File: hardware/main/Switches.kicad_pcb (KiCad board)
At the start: 4 copper layers, 120 x 75 mm, 108 parts, among them J101 BusBar, J102 BusBar, J103 BusBar, J104 BusBar, J105 Conn_02x03_Odd_Even, Q101 IPT015N10N5, Q102 IPT015N10N5, Q103 IPT015N10N5, Q104 IPT015N10N5, Q105 IPT015N10N5, Q106 IPT015N10N5, Q107 IPT015N10N5, Q108 IPT015N10N5, Q109 IPT015N10N5, Q110 IPT015N10N5, Q111 IPT015N10N5, Q112 IPT015N10N5, U101 UCC27211DDAR, U102 UCC27211DDAR

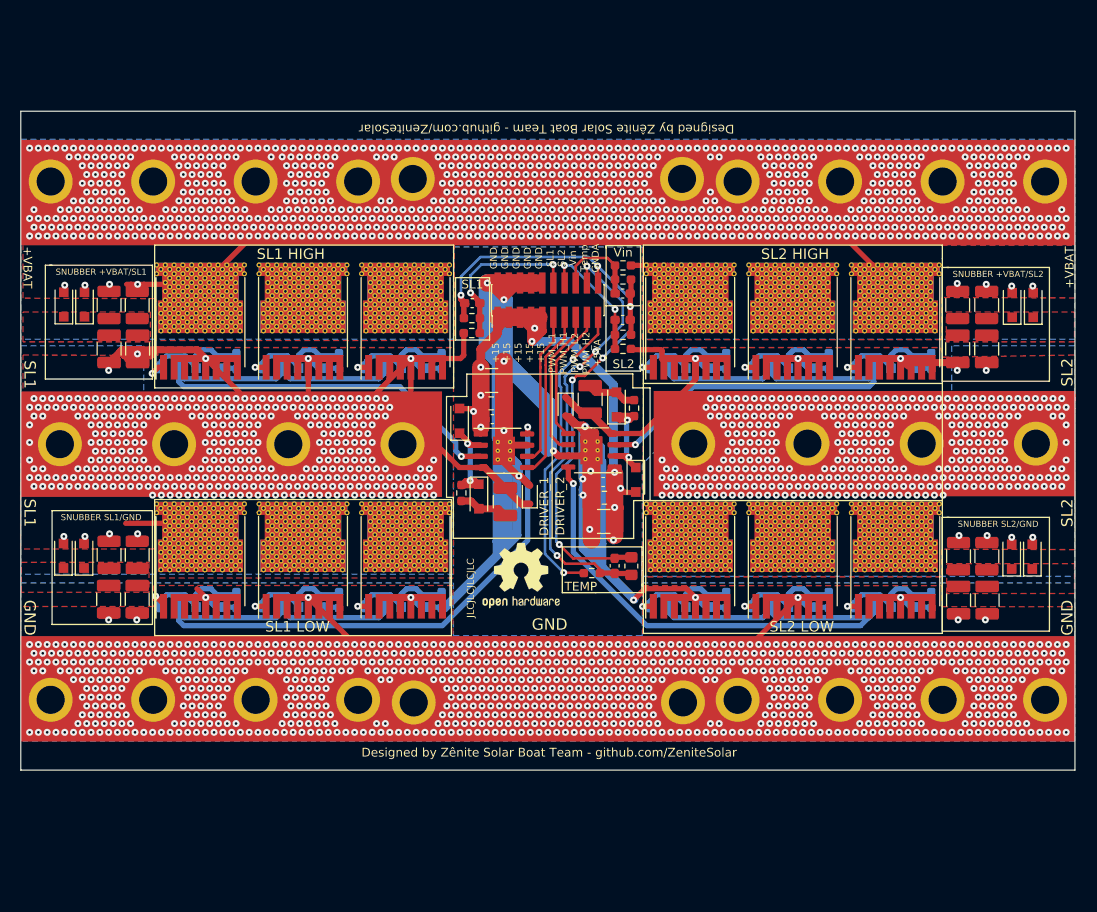
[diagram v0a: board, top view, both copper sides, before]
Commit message: board finalized
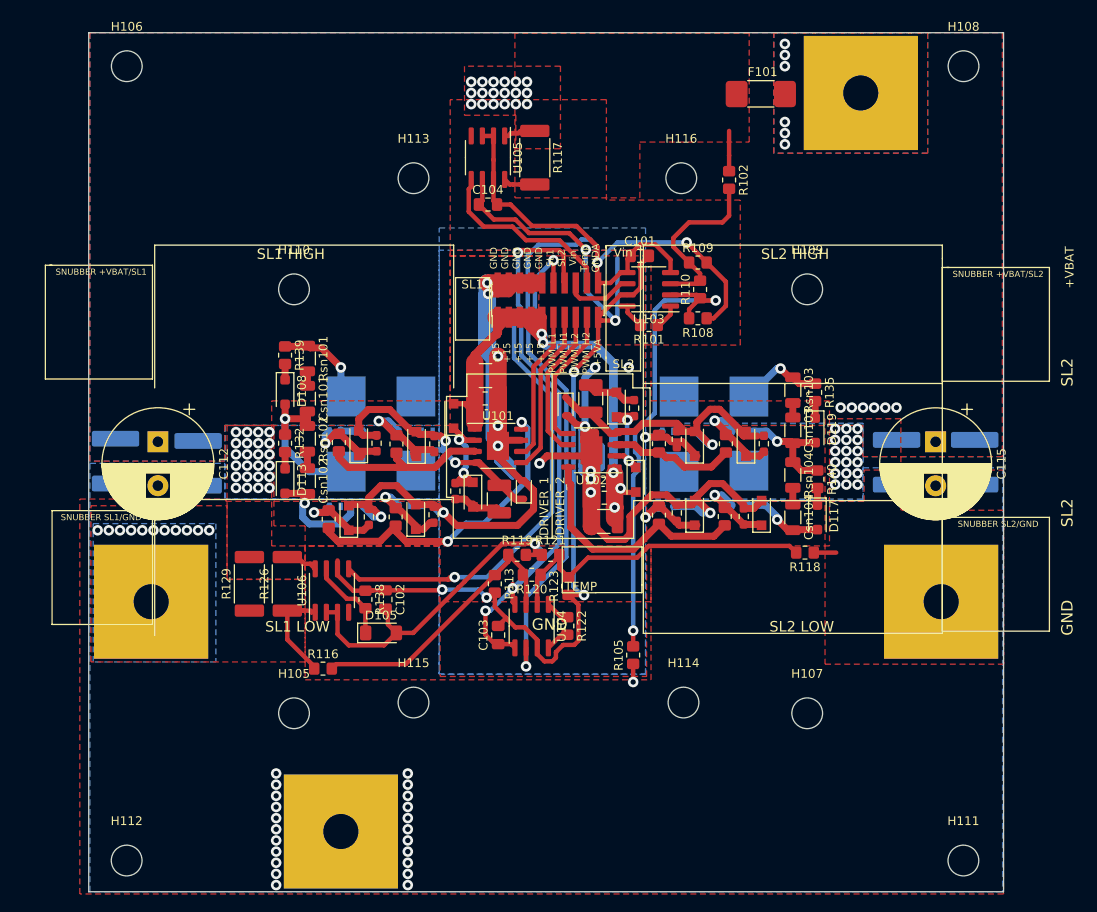
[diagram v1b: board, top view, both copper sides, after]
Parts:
- removed C131, C132, C133: 1n, Capacitor_SMD:C_0603_1608Metric_Pad1.08x0.95mm_HandSolder
- removed C134: 100n, Capacitor_SMD:C_0603_1608Metric_Pad1.08x0.95mm_HandSolder
- removed Csn105, Csn107: 100n, Capacitor_SMD:C_1210_3225Metric_Pad1.33x2.70mm_HandSolder
- removed Csn106, Csn108: NC, Capacitor_SMD:C_1210_3225Metric_Pad1.33x2.70mm_HandSolder
- removed Dsn101, Dsn103, Dsn105, Dsn107: MBR2H100SFT3G, Diode_SMD:D_SOD-123F
- removed Dsn102, Dsn104, Dsn106, Dsn108: NC, Diode_SMD:D_SOD-123F
- removed J101, J102: BusBar, Switches:BusBar1
- removed J103, J104: BusBar, Switches:BusBar2
- removed Q103, Q106, Q109, Q112: IPT015N10N5, Switches:Infineon_PG-HSOF-8-1_ThermalVias3
- removed REF**: OSHW-Logo2_9.8x8mm_SilkScreen, Symbol:OSHW-Logo2_9.8x8mm_SilkScreen
- removed Rsn105, Rsn107: 10, Resistor_SMD:R_1210_3225Metric_Pad1.30x2.65mm_HandSolder
- removed Rsn106, Rsn108: NC, Resistor_SMD:R_1210_3225Metric_Pad1.30x2.65mm_HandSolder
- removed TH101: SDNT2012X103F3950FTF, Resistor_SMD:R_0805_2012Metric_Pad1.20x1.40mm_HandSolder
- added C101: 100n, Capacitor_SMD:C_0805_2012Metric_Pad1.18x1.45mm_HandSolder, F.Cu at (172.7, 80.0)
- added C102: 100n, Capacitor_SMD:C_0805_2012Metric_Pad1.18x1.45mm_HandSolder, F.Cu at (143.8, 119.1)
- added C103: 100n, Capacitor_SMD:C_0805_2012Metric_Pad1.18x1.45mm_HandSolder, F.Cu at (156.6, 123.2)
- added C104: 100n, Capacitor_SMD:C_0805_2012Metric_Pad1.18x1.45mm_HandSolder, F.Cu at (155.4, 74.2)
- added C112: 80V 4700uF, Capacitor_THT:CP_Radial_D12.5mm_P5.00mm, F.Cu at (117.9, 101.2)
- added C115: 80V 4700uF, Capacitor_THT:CP_Radial_D12.5mm_P5.00mm, F.Cu at (206.4, 101.2)
- added Cc101: 250V 1uF X7R ±10% 20mR 2220, Capacitor_SMD:C_2220_5650Metric, B.Cu at (201.9, 103.5)
- added Cc102: 250V 1uF X7R ±10% 20mR 2220, Capacitor_SMD:C_2220_5650Metric, B.Cu at (210.8, 103.5)
- added Cc103: 250V 1uF X7R ±10% 20mR 2220, Capacitor_SMD:C_2220_5650Metric, B.Cu at (122.4, 103.6)
- added Cc104: 250V 1uF X7R ±10% 20mR 2220, Capacitor_SMD:C_2220_5650Metric, B.Cu at (113.0, 103.4)
- added D119: SMF100A, Diode_SMD:D_SOD-123F, F.Cu at (192.7, 99.9)
- added F101: 65V 20A 3mOhms Fuse, Zenite:S6125-F, F.Cu at (186.7, 61.5)
- added H101: Vin+, Zenite:MountingHole_13mmx13mm_Rectangular, F.Cu at (197.9, 61.5)
- added H102: Vin-, Zenite:MountingHole_13mmx13mm_Rectangular, F.Cu at (138.7, 145.5)
- added H103: Vout-, Zenite:MountingHole_13mmx13mm_Rectangular, F.Cu at (207.0, 119.4)
- added H104: Vout+, Zenite:MountingHole_13mmx13mm_Rectangular, F.Cu at (117.1, 119.4)
- added H105: MountingHole, MountingHole:MountingHole_3.5mm, F.Cu at (133.3, 132.1)
- added H106: MountingHole, MountingHole:MountingHole_3.5mm, F.Cu at (114.3, 58.4)
- added H107: MountingHole, MountingHole:MountingHole_3.5mm, F.Cu at (191.8, 132.1)
- added H108: MountingHole, MountingHole:MountingHole_3.5mm, F.Cu at (209.6, 58.4)
- added H109: MountingHole, MountingHole:MountingHole_3.5mm, F.Cu at (191.8, 83.8)
- added H110: MountingHole, MountingHole:MountingHole_3.5mm, F.Cu at (133.3, 83.8)
- added H111: MountingHole, MountingHole:MountingHole_3.5mm, F.Cu at (209.6, 148.8)
- added H112: MountingHole, MountingHole:MountingHole_3.5mm, F.Cu at (114.3, 148.8)
- added H113: MountingHole, MountingHole:MountingHole_3.5mm, F.Cu at (147.0, 71.2)
- added H114: MountingHole, MountingHole:MountingHole_3.5mm, F.Cu at (177.7, 130.9)
- added H115: MountingHole, MountingHole:MountingHole_3.5mm, F.Cu at (147.0, 130.9)
- added H116: MountingHole, MountingHole:MountingHole_3.5mm, F.Cu at (177.4, 71.2)
- added R101: ?, Resistor_SMD:R_0805_2012Metric_Pad1.20x1.40mm_HandSolder, F.Cu at (173.8, 87.9)
- added R102: ?, Resistor_SMD:R_0805_2012Metric_Pad1.20x1.40mm_HandSolder, F.Cu at (182.9, 71.4)
- added R109: ?, Resistor_SMD:R_0805_2012Metric_Pad1.20x1.40mm_HandSolder, F.Cu at (179.3, 80.8)
- added R110: ?, Resistor_SMD:R_0805_2012Metric_Pad1.20x1.40mm_HandSolder, F.Cu at (179.6, 83.8)
- added R138: 1k, Resistor_SMD:R_0805_2012Metric_Pad1.20x1.40mm_HandSolder, F.Cu at (141.5, 119.1)
- added R139: 0R, Resistor_SMD:R_0805_2012Metric_Pad1.20x1.40mm_HandSolder, F.Cu at (132.3, 91.3)
- added R140: 0R, Resistor_SMD:R_0805_2012Metric_Pad1.20x1.40mm_HandSolder, F.Cu at (192.9, 105.4)
- added U103: INA823, Package_SO:SOIC-8_3.9x4.9mm_P1.27mm, F.Cu at (173.7, 83.8)
- added U104: INA823, Package_SO:SOIC-8_3.9x4.9mm_P1.27mm, F.Cu at (160.4, 122.2)
- added U105: INA283, Package_SO:SOIC-8_3.9x4.9mm_P1.27mm, F.Cu at (155.4, 68.8)
- added U106: INA283, Package_SO:SOIC-8_3.9x4.9mm_P1.27mm, F.Cu at (137.7, 118.1)
- Csn101, Csn103: footprint Capacitor_SMD:C_1210_3225Metric_Pad1.33x2.70mm_HandSolder -> Resistor_SMD:R_1206_3216Metric
- Csn102, Csn104: value NC -> 100n; footprint Capacitor_SMD:C_1210_3225Metric_Pad1.33x2.70mm_HandSolder -> Resistor_SMD:R_1206_3216Metric
- D101, D104, D106, D107, D109, D112, D115, D116, R103, R104, R106, R107, R111, R112, R114, R115, R124, R125, R127, R128, R130, R131, R133, R134: moved to F.Cu
- D105: value B0530W -> 3v6; footprint Diode_SMD:D_SOD-123F -> Diode_SMD:D_MiniMELF; moved to F.Cu
- D108, D113, D117: value B0530W -> SMF100A; moved to F.Cu
- Q101, Q102, Q104, Q105, Q107, Q108, Q110, Q111: value IPT015N10N5 -> BSC093N15NS5; footprint Switches:Infineon_PG-HSOF-8-1_ThermalVias3 -> Zenite:TDSON-8-3; moved to B.Cu
- R105, R108, R113, R116: value 4R7 -> ?; moved to F.Cu
- R117: value 5k6 -> 1.0mR 1% 5W 50ppm; footprint Resistor_SMD:R_0603_1608Metric_Pad0.98x0.95mm_HandSolder -> Resistor_SMD:R_2512_6332Metric_Pad1.40x3.35mm_HandSolder
- R118, R119, R120: value 10k -> ?; footprint Resistor_SMD:R_0603_1608Metric_Pad0.98x0.95mm_HandSolder -> Resistor_SMD:R_0805_2012Metric_Pad1.20x1.40mm_HandSolder
- R121: value 330 -> ?; footprint Resistor_SMD:R_0603_1608Metric_Pad0.98x0.95mm_HandSolder -> Resistor_SMD:R_0805_2012Metric_Pad1.20x1.40mm_HandSolder
- R122, R123: value 3k3 -> ?; footprint Resistor_SMD:R_0603_1608Metric_Pad0.98x0.95mm_HandSolder -> Resistor_SMD:R_0805_2012Metric_Pad1.20x1.40mm_HandSolder
- R126, R129: value 10k -> 1.0mR 1% 5W 50ppm; footprint Resistor_SMD:R_0603_1608Metric_Pad0.98x0.95mm_HandSolder -> Resistor_SMD:R_2512_6332Metric_Pad1.40x3.35mm_HandSolder; moved to F.Cu
- R132, R135: value 10k -> 0R; footprint Resistor_SMD:R_0603_1608Metric_Pad0.98x0.95mm_HandSolder -> Resistor_SMD:R_0805_2012Metric_Pad1.20x1.40mm_HandSolder; moved to F.Cu
- Rsn101, Rsn103: footprint Resistor_SMD:R_1210_3225Metric_Pad1.30x2.65mm_HandSolder -> Resistor_SMD:R_1206_3216Metric
- Rsn102, Rsn104: value NC -> 10; footprint Resistor_SMD:R_1210_3225Metric_Pad1.30x2.65mm_HandSolder -> Resistor_SMD:R_1206_3216Metric
- U101, U102: footprint Switches:SOIC-8-1EP_3.9x4.9mm_P1.27mm_EP2.514x3.2mm_ThermalVias -> Package_SO:SOIC-8-1EP_3.9x4.9mm_P1.27mm_EP2.514x3.2mm
- moved R132 74.2 mm to (132.3, 101.3), turned to -90 degrees
- moved D113 71.5 mm to (132.3, 105.6), turned to -90 degrees
- moved R116 62.1 mm to (136.7, 127.0)
- moved R108 49.2 mm to (179.3, 87.1), turned to 180 degrees
- moved R113 48.8 mm to (156.2, 117.3), turned to -90 degrees
- moved R117 47.7 mm to (160.8, 68.8), turned to -90 degrees
- moved R118 45.4 mm to (191.5, 113.8), turned to 180 degrees
- moved R105 44.0 mm to (172.0, 125.5), turned to 90 degrees
- moved R120 36.7 mm to (160.4, 116.3)
- moved R123 35.4 mm to (164.6, 117.6), turned to 90 degrees
- moved R122 33.7 mm to (164.5, 122.1), turned to -90 degrees
- moved R126 30.8 mm to (132.6, 117.3)
- moved D105 30.4 mm to (143.3, 122.9)
- moved Rsn104 29.3 mm to (190.1, 105.0)
- moved Csn104 29.2 mm to (190.1, 109.8)
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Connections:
- Csn102 pad 1: Net-(Csn101-Pad1) -> Net-(Csn102-Pad1)
- Csn102 pad 2: /SL1 -> GND
- Csn104 pad 1: Net-(Csn103-Pad1) -> Net-(Csn104-Pad1)
- Csn104 pad 2: /SL2 -> GND
- D105 pad 1: /GH1_3 -> Net-(D105-K)
- D105 pad 2: /SL1 -> GNDA
- D108 pad 1: /GL1_3 -> Net-(D108-A1)
- D108 pad 2: GND -> /SL1
- D113 pad 1: /GH2_3 -> Net-(D113-A1)
- D113 pad 2: /SL2 -> GND
- D117 pad 1: /GL3_3 -> Net-(D117-A1)
- J105 pad 12: /SL1_sen -> /Vout_Sense
- J105 pad 14: /SL2_sen -> /Iout_Sense
- J105 pad 16: /Vin_sen -> /Vin_Sense
- J105 pad 18: /TEMP1 -> /Iin_Sense
- Q101 pad 2: /SL1 -> +BATT
- Q101 pad 3: +BATT -> /SL1
- Q102 pad 2: /SL1 -> +BATT
- Q102 pad 3: +BATT -> /SL1
- Q104 pad 2: /SL2 -> +BATT
- Q104 pad 3: +BATT -> /SL2
- Q105 pad 2: /SL2 -> +BATT
- Q105 pad 3: +BATT -> /SL2
- Q107 pad 2: GND -> /SL1
- Q107 pad 3: /SL1 -> GND
- Q108 pad 2: GND -> /SL1
- Q108 pad 3: /SL1 -> GND
- Q110 pad 2: GND -> /SL2
- Q110 pad 3: /SL2 -> GND
- Q111 pad 2: GND -> /SL2
- Q111 pad 3: /SL2 -> GND
- R103 pad 2: Net-(R103-Pad2) -> Net-(U101-HO)
- R104 pad 2: Net-(R103-Pad2) -> Net-(U101-HO)
- R105 pad 1: /GH1_3 -> GND
- R105 pad 2: Net-(R103-Pad2) -> Net-(U103--)
- R106 pad 2: Net-(R106-Pad2) -> Net-(U101-LO)
- R107 pad 2: Net-(R106-Pad2) -> Net-(U101-LO)
- R108 pad 1: /GL1_3 -> GNDA
- R108 pad 2: Net-(R106-Pad2) -> Net-(U103--)
- R111 pad 2: Net-(R111-Pad2) -> Net-(U102-HO)
- R112 pad 2: Net-(R111-Pad2) -> Net-(U102-HO)
- R113 pad 1: /GH2_3 -> Net-(U104-+)
- R113 pad 2: Net-(R111-Pad2) -> +5VA
- R114 pad 2: Net-(R114-Pad2) -> Net-(U102-LO)
- R115 pad 2: Net-(R114-Pad2) -> Net-(U102-LO)
- R116 pad 1: /GL3_3 -> /Vout+
- R116 pad 2: Net-(R114-Pad2) -> Net-(U104-+)
- R117 pad 1: +5VA -> +BATT
- R117 pad 2: /TEMP1 -> /Vbat+_Fus
- R118 pad 1: /SL1 -> /SL2
- R118 pad 2: /SL1_sen -> Net-(U104--)
- R119 pad 1: /SL2 -> Net-(U104-+)
- R119 pad 2: /SL2_sen -> GNDA
- R120 pad 1: +BATT -> Net-(U104--)
- R120 pad 2: /Vin_sen -> Net-(U104-+)
- R121 pad 1: /SL1_sen -> GNDA
- R121 pad 2: GNDA -> Net-(U104--)
- R122 pad 1: /SL2_sen -> Net-(R122-Pad1)
- R122 pad 2: GNDA -> Net-(R122-Pad2)
- R123 pad 1: /Vin_sen -> +5VA
- R123 pad 2: GNDA -> Net-(U104--)
- R126 pad 1: /SL1 -> /Vout+
- R126 pad 2: /GH1_3 -> /SL1
- R129 pad 1: GND -> /Vout+
- R129 pad 2: /GL1_3 -> /SL1
- R132 pad 1: /SL2 -> /SL1
- R132 pad 2: /GH2_3 -> Net-(D113-A1)
- R135 pad 1: GND -> +BATT
- R135 pad 2: /GL3_3 -> Net-(D119-A1)
- Rsn102 pad 1: +BATT -> /SL1
- Rsn102 pad 2: Net-(Csn101-Pad1) -> Net-(Csn102-Pad1)
- Rsn104 pad 1: +BATT -> /SL2
- Rsn104 pad 2: Net-(Csn103-Pad1) -> Net-(Csn104-Pad1)
- U101 pad 3: Net-(R103-Pad2) -> Net-(U101-HO)
- U101 pad 8: Net-(R106-Pad2) -> Net-(U101-LO)
- U102 pad 3: Net-(R111-Pad2) -> Net-(U102-HO)
- U102 pad 8: Net-(R114-Pad2) -> Net-(U102-LO)
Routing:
- net GND: track 392.4 -> 287.5 mm, vias 974 -> 40
- net GNDA: track 77.9 -> 176.5 mm, vias 6 -> 5
- net +5VA: track 34.9 -> 127.0 mm, vias 2 -> 6
- net Net-(R106-Pad2): track 84.8 -> 0.00 mm, vias 1 -> 0
- net +BATT: track 104.7 -> 26.1 mm, vias 961 -> 26
- net Net-(R114-Pad2): track 74.4 -> 0.00 mm, vias 1 -> 0
- net /SL1: track 125.2 -> 56.7 mm, vias 389 -> 27
- net /Iout_Sense: track 0.00 -> 67.7 mm, vias 0 -> 2
- net Net-(R103-Pad2): track 67.0 -> 0.00 mm, vias 1 -> 0
- net Net-(R111-Pad2): track 59.6 -> 0.00 mm, vias 1 -> 0
- net /Vout_Sense: track 0.00 -> 56.5 mm, vias 0 -> 2
- net Net-(U103--): track 0.00 -> 55.3 mm, vias 0 -> 2
- net /TEMP1: track 50.5 -> 0.00 mm, vias 4 -> 0
- net Net-(U104--): track 0.00 -> 38.7 mm
- net Net-(U101-LO): track 0.00 -> 36.0 mm, vias 0 -> 2
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- added copper zone on F.Cu, net /Vbat+_Fus
- added copper zone on B.Cu, net /Vbat+_Unf
- added copper zone on F.Cu, net /Vbat+_Unf
- added copper zone on B.Cu, net /Vout+
- added copper zone on F.Cu, net /Vout+
- added copper zone on F.Cu, net GNDA
- removed copper zone on In2.Cu, net +15V
- removed copper zone on In1.Cu, net +BATT
- removed copper zone on In2.Cu, net +BATT
- removed copper zone on In1.Cu, net /SL1
- removed copper zone on In2.Cu, net /SL1
- removed copper zone on In1.Cu, net /SL2
- removed copper zone on In2.Cu, net /SL2
- removed copper zone on In1.Cu, net GND
- removed copper zone on In2.Cu, net GND
- removed copper zone on F.Cu, net Net-(Csn101-Pad1)
- removed copper zone on F.Cu, net Net-(Csn103-Pad1)
- removed copper zone on F.Cu, net Net-(Csn105-Pad1)
- removed copper zone on F.Cu, net Net-(Csn107-Pad1)
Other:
- board size 120 x 75 mm -> 104.1 x 97.8 mm
- copper layers 4 -> 2
- net class Default removed
- board text removed: "Designed by Zênite Solar Boat Team - github.com/ZeniteSolar"
- board text removed: "JLCJLCJLCJLC"
